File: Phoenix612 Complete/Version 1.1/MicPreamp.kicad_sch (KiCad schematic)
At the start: 18 parts, among them J16 TP10, J17 MICIN, Q2 2N3904

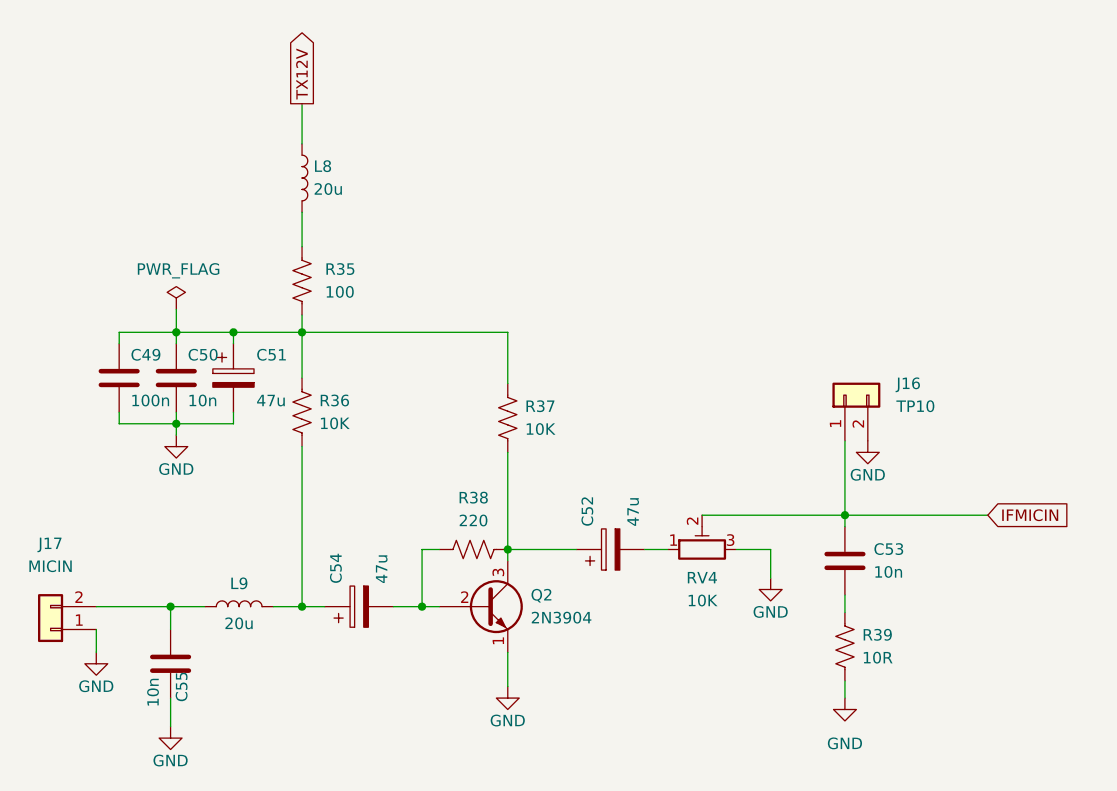
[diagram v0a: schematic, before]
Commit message: Update 24Mar23
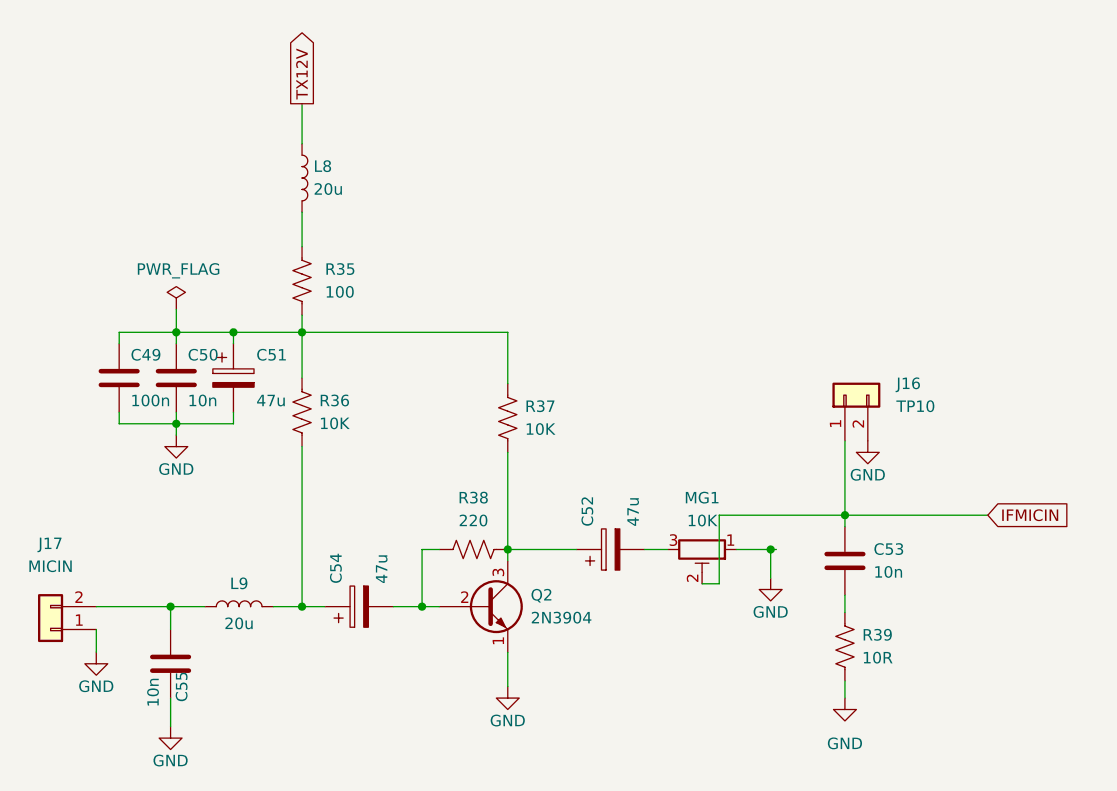
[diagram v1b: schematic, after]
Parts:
- renumbered RV4 to MG1
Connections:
- net GND: now also MG1.1; no longer MG1.3
- net at C52.2: now also MG1.3; no longer MG1.1
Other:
- moved on the sheet: MG1
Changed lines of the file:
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@@
   (junction (at 82.55 71.755) (diameter 0) (color 0 0 0 0)
   )
+  (junction (at 142.24 95.885) (diameter 0) (color 0 0 0 0)
+  )
   (junction (at 76.2 81.915) (diameter 0) (color 0 0 0 0)
   )
@@
     (stroke (width 0) (type default) (color 0 0 0 0))
   )
-  (wire (pts (xy 134.62 92.075) (xy 150.495 92.075))
-    (stroke (width 0) (type default) (color 0 0 0 0))
-  )
   (wire (pts (xy 76.2 71.755) (xy 76.2 73.025))
     (stroke (width 0) (type default) (color 0 0 0 0))
@@
     (stroke (width 0) (type default) (color 0 0 0 0))
   )
+  (wire (pts (xy 142.24 95.885) (xy 142.875 95.885))
+    (stroke (width 0) (type default) (color 0 0 0 0))
+  )
   (wire (pts (xy 67.31 102.235) (xy 75.565 102.235))
     (stroke (width 0) (type default) (color 0 0 0 0))
@@
     (stroke (width 0) (type default) (color 0 0 0 0))
   )
+  (wire (pts (xy 75.565 102.235) (xy 79.375 102.235))
+    (stroke (width 0) (type default) (color 0 0 0 0))
+  )
+  (wire (pts (xy 105.41 102.235) (xy 103.505 102.235))
+    (stroke (width 0) (type default) (color 0 0 0 0))
+  )
+  (wire (pts (xy 69.85 80.645) (xy 69.85 81.915))
+    (stroke (width 0) (type default) (color 0 0 0 0))
+  )
+  (wire (pts (xy 76.2 81.915) (xy 76.2 80.645))
+    (stroke (width 0) (type default) (color 0 0 0 0))
+  )
+  (wire (pts (xy 113.03 95.885) (xy 113.03 97.155))
+    (stroke (width 0) (type default) (color 0 0 0 0))
+  )
+  (wire (pts (xy 76.2 81.915) (xy 82.55 81.915))
+    (stroke (width 0) (type default) (color 0 0 0 0))
+  )
+  (wire (pts (xy 67.31 107.315) (xy 67.31 104.775))
+    (stroke (width 0) (type default) (color 0 0 0 0))
+  )
+  (wire (pts (xy 75.565 102.235) (xy 75.565 104.775))
+    (stroke (width 0) (type default) (color 0 0 0 0))
+  )
+  (wire (pts (xy 113.03 85.09) (xy 113.03 95.885))
+    (stroke (width 0) (type default) (color 0 0 0 0))
+  )
+  (wire (pts (xy 90.17 71.755) (xy 90.17 76.835))
+    (stroke (width 0) (type default) (color 0 0 0 0))
+  )
+  (wire (pts (xy 90.17 84.455) (xy 90.17 102.235))
+    (stroke (width 0) (type default) (color 0 0 0 0))
+  )
+  (wire (pts (xy 76.2 69.215) (xy 76.2 71.755))
+    (stroke (width 0) (type default) (color 0 0 0 0))
+  )
+  (wire (pts (xy 90.17 71.755) (xy 113.03 71.755))
+    (stroke (width 0) (type default) (color 0 0 0 0))
+  )
+  (wire (pts (xy 113.03 95.885) (xy 120.65 95.885))
+    (stroke (width 0) (type default) (color 0 0 0 0))
+  )
+  (wire (pts (xy 136.525 92.075) (xy 150.495 92.075))
+    (stroke (width 0) (type default) (color 0 0 0 0))
+  )
+  (wire (pts (xy 82.55 71.755) (xy 82.55 73.025))
+    (stroke (width 0) (type default) (color 0 0 0 0))
+  )
+  (wire (pts (xy 134.62 99.695) (xy 136.525 99.695))
+    (stroke (width 0) (type default) (color 0 0 0 0))
+  )
+  (wire (pts (xy 103.505 95.885) (xy 103.505 102.235))
+    (stroke (width 0) (type default) (color 0 0 0 0))
+  )
+  (wire (pts (xy 86.995 102.235) (xy 90.17 102.235))
+    (stroke (width 0) (type default) (color 0 0 0 0))
+  )
+  (wire (pts (xy 92.71 102.235) (xy 90.17 102.235))
+    (stroke (width 0) (type default) (color 0 0 0 0))
+  )
+  (wire (pts (xy 69.85 71.755) (xy 76.2 71.755))
+    (stroke (width 0) (type default) (color 0 0 0 0))
+  )
+  (wire (pts (xy 150.495 92.075) (xy 166.37 92.075))
+    (stroke (width 0) (type default) (color 0 0 0 0))
+  )
+  (wire (pts (xy 75.565 115.57) (xy 75.565 112.395))
+    (stroke (width 0) (type default) (color 0 0 0 0))
+  )
+  (wire (pts (xy 69.85 81.915) (xy 76.2 81.915))
+    (stroke (width 0) (type default) (color 0 0 0 0))
+  )
+  (wire (pts (xy 136.525 99.695) (xy 136.525 92.075))
+    (stroke (width 0) (type default) (color 0 0 0 0))
+  )
   (wire (pts (xy 138.43 95.885) (xy 142.24 95.885))
     (stroke (width 0) (type default) (color 0 0 0 0))
   )
-  (wire (pts (xy 75.565 102.235) (xy 79.375 102.235))
-    (stroke (width 0) (type default) (color 0 0 0 0))
-  )
-  (wire (pts (xy 105.41 102.235) (xy 103.505 102.235))
-    (stroke (width 0) (type default) (color 0 0 0 0))
-  )
-  (wire (pts (xy 69.85 80.645) (xy 69.85 81.915))
-    (stroke (width 0) (type default) (color 0 0 0 0))
-  )
-  (wire (pts (xy 76.2 81.915) (xy 76.2 80.645))
-    (stroke (width 0) (type default) (color 0 0 0 0))
-  )
-  (wire (pts (xy 113.03 95.885) (xy 113.03 97.155))
-    (stroke (width 0) (type default) (color 0 0 0 0))
-  )
-  (wire (pts (xy 76.2 81.915) (xy 82.55 81.915))
-    (stroke (width 0) (type default) (color 0 0 0 0))
-  )
-  (wire (pts (xy 67.31 107.315) (xy 67.31 104.775))
-    (stroke (width 0) (type default) (color 0 0 0 0))
-  )
-  (wire (pts (xy 75.565 102.235) (xy 75.565 104.775))
-    (stroke (width 0) (type default) (color 0 0 0 0))
-  )
-  (wire (pts (xy 113.03 85.09) (xy 113.03 95.885))
-    (stroke (width 0) (type default) (color 0 0 0 0))
-  )
-  (wire (pts (xy 90.17 71.755) (xy 90.17 76.835))
-    (stroke (width 0) (type default) (color 0 0 0 0))
-  )
-  (wire (pts (xy 90.17 84.455) (xy 90.17 102.235))
-    (stroke (width 0) (type default) (color 0 0 0 0))
-  )
-  (wire (pts (xy 76.2 69.215) (xy 76.2 71.755))
-    (stroke (width 0) (type default) (color 0 0 0 0))
-  )
-  (wire (pts (xy 90.17 71.755) (xy 113.03 71.755))
-    (stroke (width 0) (type default) (color 0 0 0 0))
-  )
-  (wire (pts (xy 113.03 95.885) (xy 120.65 95.885))
-    (stroke (width 0) (type default) (color 0 0 0 0))
-  )
-  (wire (pts (xy 82.55 71.755) (xy 82.55 73.025))
-    (stroke (width 0) (type default) (color 0 0 0 0))
-  )
-  (wire (pts (xy 103.505 95.885) (xy 103.505 102.235))
-    (stroke (width 0) (type default) (color 0 0 0 0))
-  )
-  (wire (pts (xy 86.995 102.235) (xy 90.17 102.235))
-    (stroke (width 0) (type default) (color 0 0 0 0))
-  )
-  (wire (pts (xy 92.71 102.235) (xy 90.17 102.235))
-    (stroke (width 0) (type default) (color 0 0 0 0))
-  )
-  (wire (pts (xy 69.85 71.755) (xy 76.2 71.755))
-    (stroke (width 0) (type default) (color 0 0 0 0))
-  )
-  (wire (pts (xy 130.81 95.885) (xy 128.27 95.885))
-    (stroke (width 0) (type default) (color 0 0 0 0))
-  )
-  (wire (pts (xy 150.495 92.075) (xy 166.37 92.075))
-    (stroke (width 0) (type default) (color 0 0 0 0))
-  )
-  (wire (pts (xy 75.565 115.57) (xy 75.565 112.395))
-    (stroke (width 0) (type default) (color 0 0 0 0))
-  )
-  (wire (pts (xy 69.85 81.915) (xy 76.2 81.915))
-    (stroke (width 0) (type default) (color 0 0 0 0))
-  )
   (wire (pts (xy 76.2 81.915) (xy 76.2 83.185))
     (stroke (width 0) (type default) (color 0 0 0 0))
   )
   (wire (pts (xy 105.41 95.885) (xy 103.505 95.885))
+    (stroke (width 0) (type default) (color 0 0 0 0))
+  )
+  (wire (pts (xy 128.27 95.885) (xy 130.81 95.885))
     (stroke (width 0) (type default) (color 0 0 0 0))
   )
@@
     (pin "2")
   )
-  (symbol (lib_id "Device:R_Potentiometer_Trim") (at 134.62 95.885 90) (unit 1)
-    (in_bom yes) (on_board yes) (fields_autoplaced)
-    (property "Reference" "RV4" (id 0) (at 134.62 99.06 90))
-    (property "Value" "10K" (id 1) (at 134.62 101.6 90))
+  (symbol (lib_id "Device:R_Potentiometer_Trim") (at 134.62 95.885 270) (unit 1)
+    (in_bom yes) (on_board yes) (fields_autoplaced)
+    (property "Reference" "MG1" (id 0) (at 134.62 90.17 90))
+    (property "Value" "10K" (id 1) (at 134.62 92.71 90))
     (property "Footprint" "Potentiometer_THT:Potentiometer_Bourns_3296W_Vertical" (id 2) (at 134.62 95.885 0)
       (effects (font (size 1.27 1.27)) hide)
